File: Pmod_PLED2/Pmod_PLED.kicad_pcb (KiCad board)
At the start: 2 copper layers, 74.5 x 20.3 mm, 10 parts, among them IC1 TBD62064APG, J1 Barrel_Jack_Switch, J2 Conn_01x06_Pin, J3 Conn_01x03_Pin, U1 AMS1117-3.3

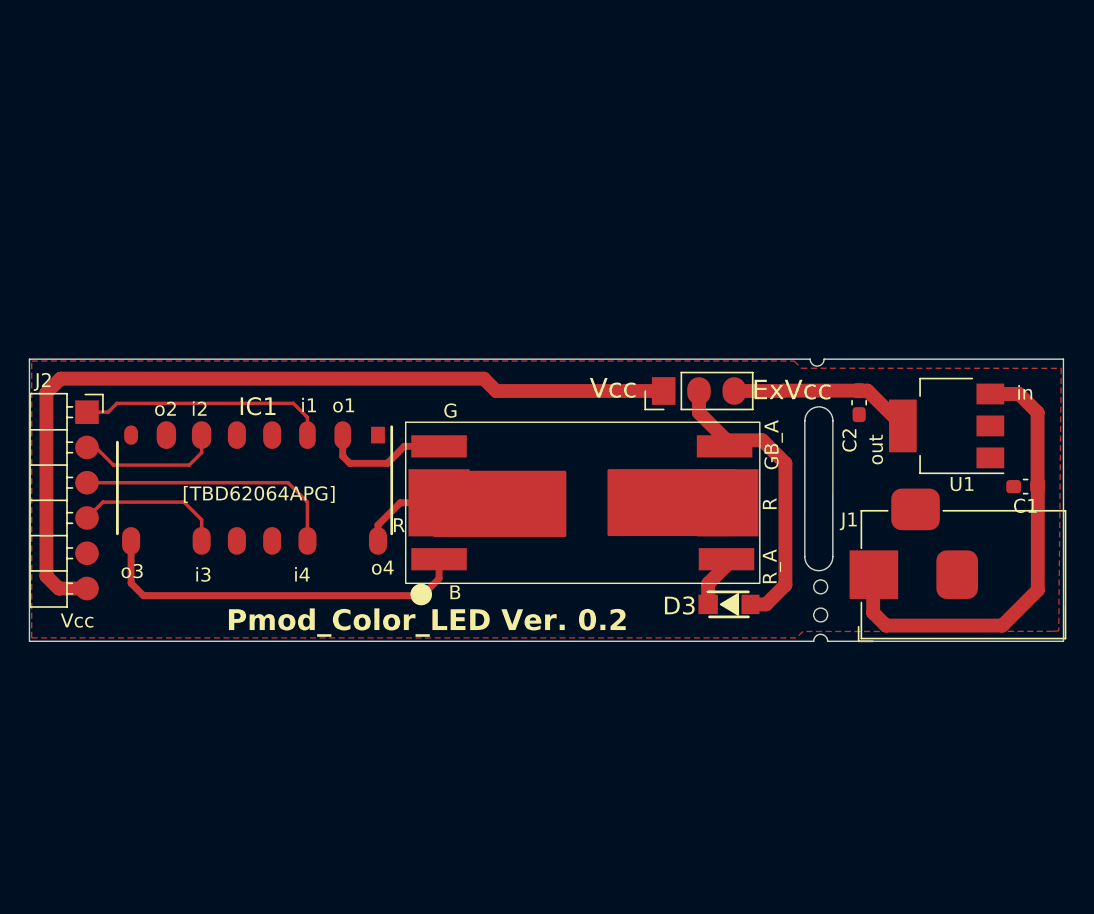
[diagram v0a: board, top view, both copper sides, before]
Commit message: power led 2 schematics
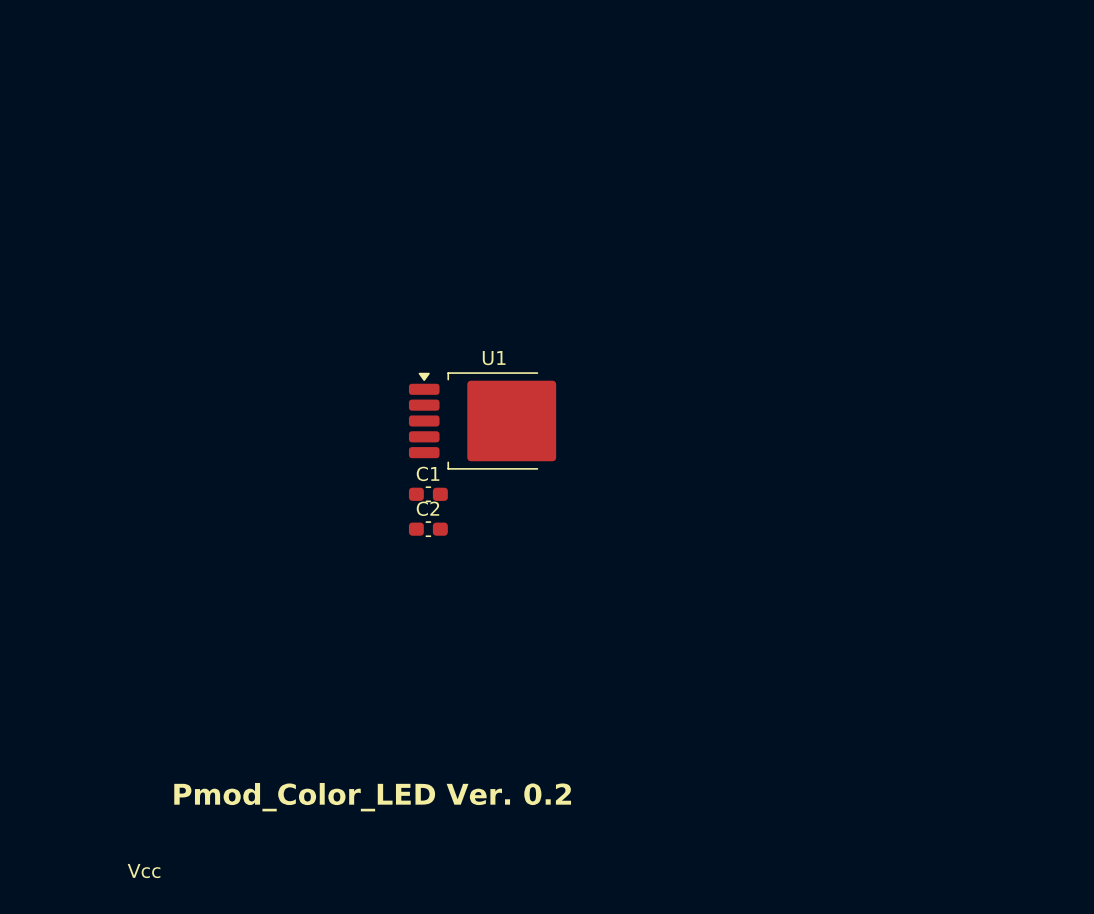
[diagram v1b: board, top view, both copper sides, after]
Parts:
- removed D1: EP204K-150G1R1B1-CA, MyLibrary:EP204-150G1R1B1-CA
- removed D3: SS2040FL, SamacSys_Parts:SODFL3618X108N
- removed G***: LOGO, MyLibrary:logo_kamo_ss
- removed IC1: TBD62064APG, SamacSys_Parts:DIP762W60P254L1975H445Q16N
- removed J1: Barrel_Jack_Switch, Connector_BarrelJack:BarrelJack_Horizontal
- removed J2: Conn_01x06_Pin, Library:Pmod6
- removed J3: Conn_01x03_Pin, Connector_PinHeader_2.54mm:PinHeader_1x03_P2.54mm_Vertical
- U1: value AMS1117-3.3 -> NJW4617; footprint Package_TO_SOT_SMD:SOT-223-3_TabPin2 -> Package_TO_SOT_SMD:TO-252-5_TabPin3
- moved C1 43.0 mm to (117.2, 85.8), turned to 0 degrees
- moved U1 32.6 mm to (121.9, 80.5), turned to 0 degrees
- moved C2 32.3 mm to (117.2, 88.3), turned to 0 degrees
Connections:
- C1 pad 1: Net-(U1-VI) -> unconnected-(C1-Pad1)
- C2 pad 2: /ExVcc -> unconnected-(C2-Pad2)
- U1 pad 1: GND -> unconnected-(U1-VDD-Pad1)
- U1 pad 2: /ExVcc -> unconnected-(U1-EN/PWM-Pad2)
- U1 pad 3: Net-(U1-VI) -> unconnected-(U1-GND-Pad3)
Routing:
- net vcc: track 61.7 -> 0.00 mm
- net Net-(U1-VI): track 32.8 -> 0.00 mm
- net Net-(D1-BK): track 26.8 -> 0.00 mm
- net /Anode: track 21.2 -> 0.00 mm
- net i4: track 19.4 -> 0.00 mm
- net i1: track 17.8 -> 0.00 mm
- net /ExVcc: track 13.2 -> 0.00 mm
- net i3: track 11.0 -> 0.00 mm
- net i2: track 10.4 -> 0.00 mm
- net Net-(D1-GK): track 9.18 -> 0.00 mm
- net Net-(IC1-O4): track 6.20 -> 0.00 mm
- net Net-(D1-RA): track 3.37 -> 0.00 mm
- removed copper zone on F.Cu, net GND
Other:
- board outline removed
- board text removed: "1"
- board text removed: "2"
- board text removed: "3"
- board text removed: "4"
- board text removed: "ExVcc"
- board text removed: "GND"
- board text removed: "[AZ1117 CH-3.3]"
- board text removed: "[TBD62064APG]"
- board text removed: "i1"
- board text removed: "i2"
- board text removed: "i3"
- board text removed: "i4"
- board text removed: "in"
- board text removed: "o1"
- board text removed: "o2"
- board text removed: "o3"
- board text removed: "o4"
- board text removed: "out"

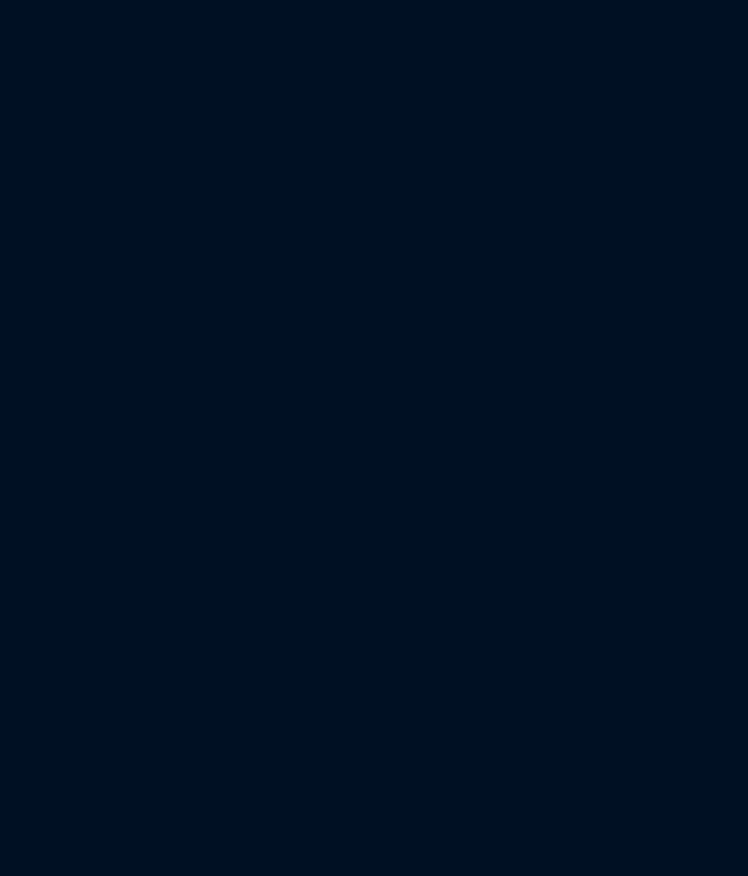
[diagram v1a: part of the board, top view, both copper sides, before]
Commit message: schematcis
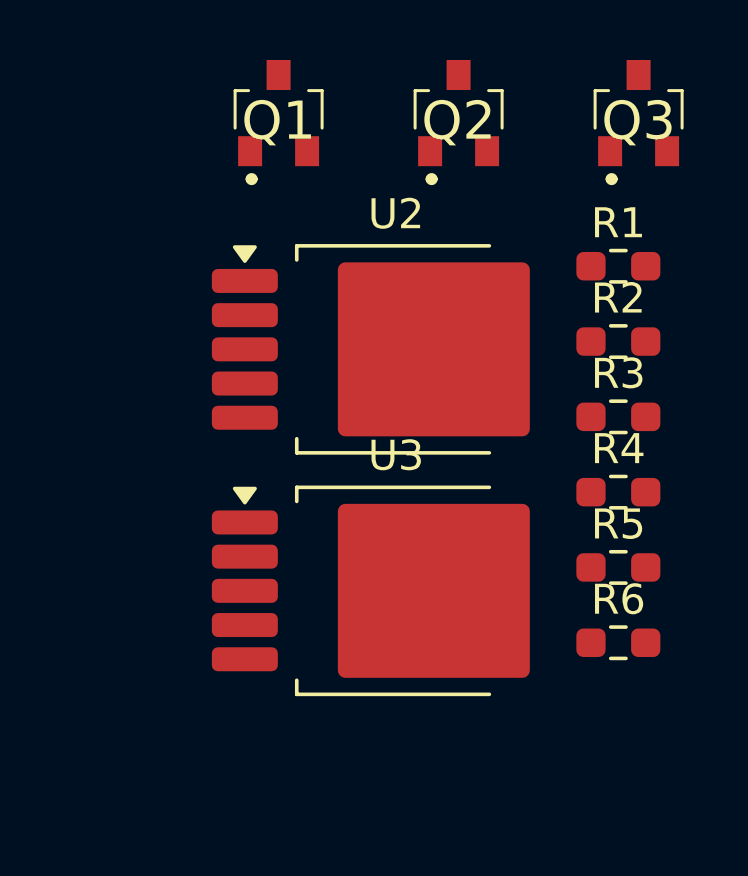
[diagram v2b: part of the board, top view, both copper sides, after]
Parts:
- added Q1: 2SC2712-BL_F_, samacsys:RN1402LF, F.Cu at (140.7, 54.5)
- added Q2: 2SC2712-BL_F_, samacsys:RN1402LF, F.Cu at (146.7, 54.5)
- added Q3: 2SC2712-BL_F_, samacsys:RN1402LF, F.Cu at (152.7, 54.5)
- added R1: 10, Resistor_SMD:R_0603_1608Metric_Pad0.98x0.95mm_HandSolder, F.Cu at (152.0, 59.1)
- added R2: 10, Resistor_SMD:R_0603_1608Metric_Pad0.98x0.95mm_HandSolder, F.Cu at (152.0, 61.6)
- added R3: 10, Resistor_SMD:R_0603_1608Metric_Pad0.98x0.95mm_HandSolder, F.Cu at (152.0, 64.1)
- added R4: 10k, Resistor_SMD:R_0603_1608Metric_Pad0.98x0.95mm_HandSolder, F.Cu at (152.0, 66.6)
- added R5: 10k, Resistor_SMD:R_0603_1608Metric_Pad0.98x0.95mm_HandSolder, F.Cu at (152.0, 69.1)
- added R6: 10k, Resistor_SMD:R_0603_1608Metric_Pad0.98x0.95mm_HandSolder, F.Cu at (152.0, 71.6)
- added U2: NJW4617, Package_TO_SOT_SMD:TO-252-5_TabPin3, F.Cu at (144.6, 61.8)
- added U3: NJW4617, Package_TO_SOT_SMD:TO-252-5_TabPin3, F.Cu at (144.6, 69.9)
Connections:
- U1 pad 1: unconnected-(U1-VDD-Pad1) -> /VCC
- U1 pad 2: unconnected-(U1-EN/PWM-Pad2) -> Net-(Q1-C)
- U1 pad 3: unconnected-(U1-GND-Pad3) -> GND
- U1 pad 4: unconnected-(U1-Rs-Pad4) -> Net-(U1-Rs)
- U1 pad 5: unconnected-(U1-LED-Pad5) -> /Anode_R
